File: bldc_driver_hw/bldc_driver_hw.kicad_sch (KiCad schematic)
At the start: 4 parts, among them J1 USB_C_Receptacle_USB2.0_16P, J2 Conn_01x03_Pin

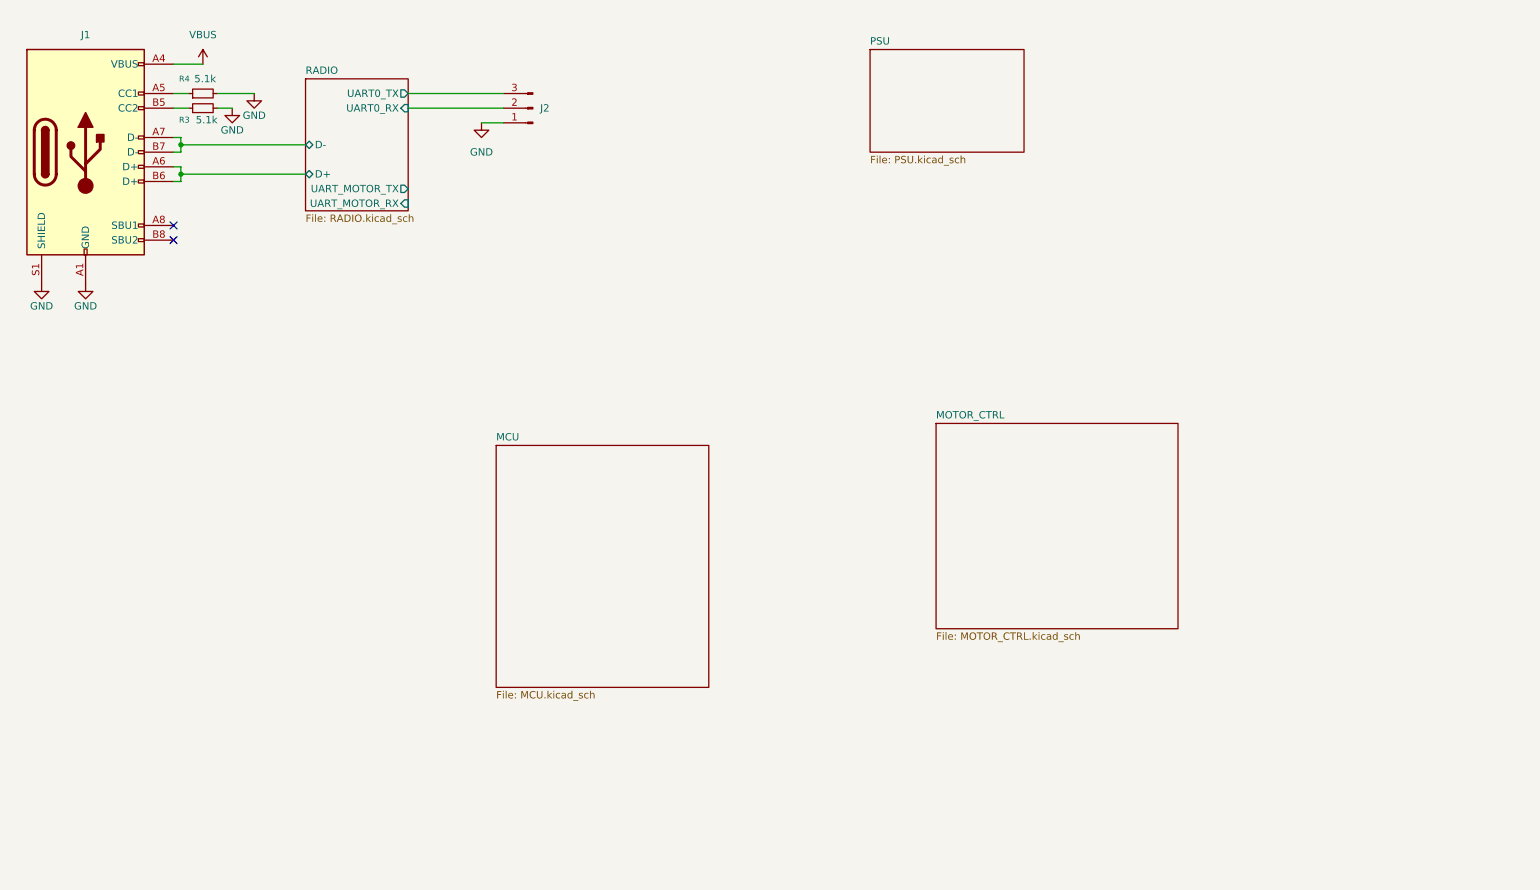
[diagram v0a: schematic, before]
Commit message: wip
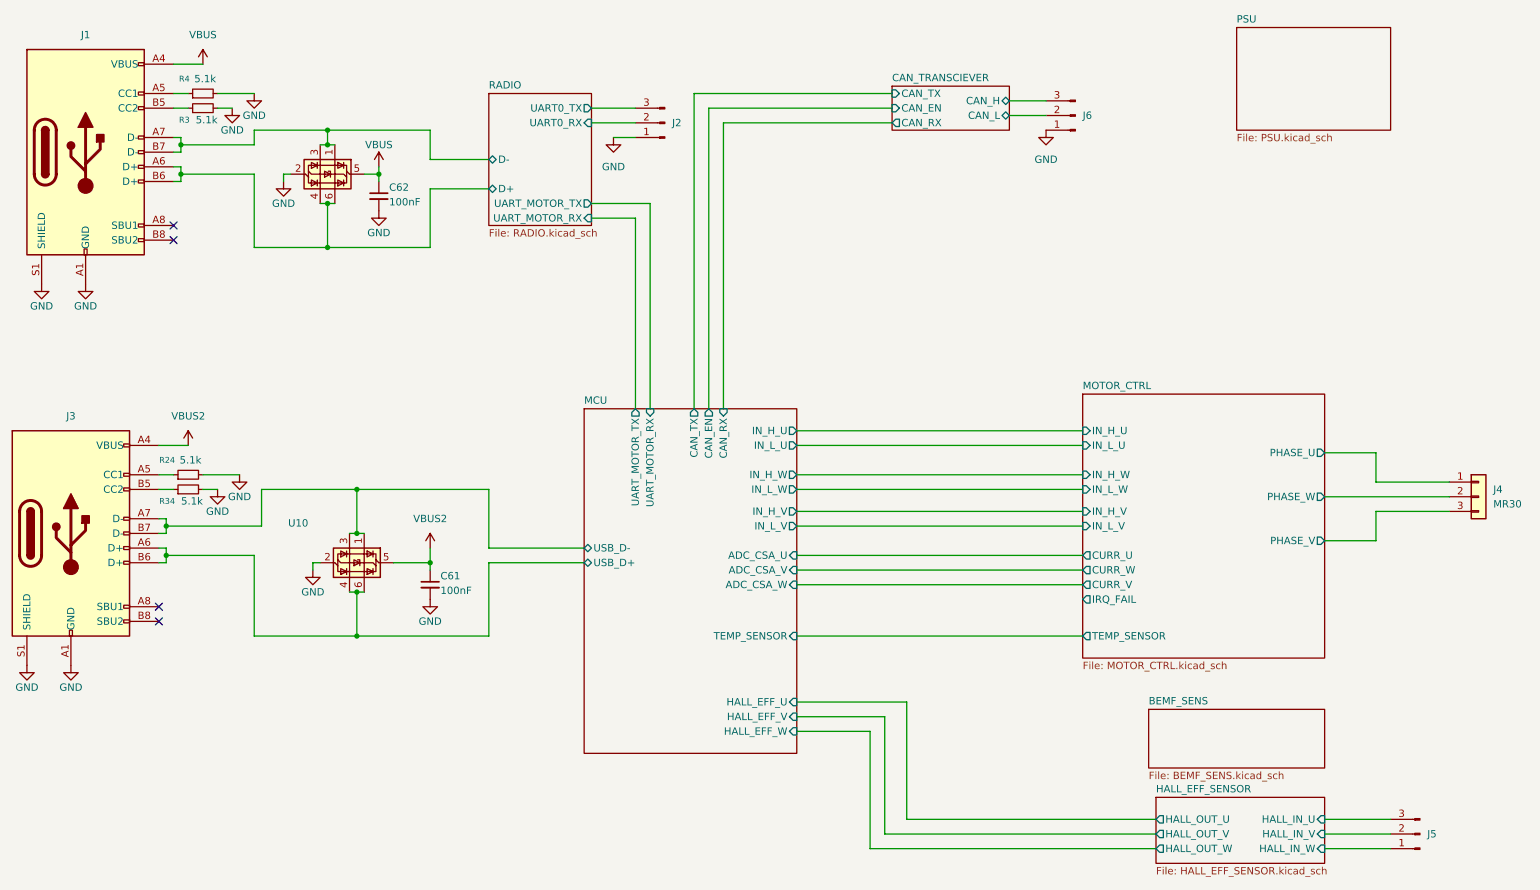
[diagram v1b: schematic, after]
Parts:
- added C61, C62: 100nF, Capacitor_SMD:C_0603_1608Metric, symbol Device:C_Small
- added J3: USB_C_Receptacle_USB2.0_16P, Connector_USB:USB_C_Receptacle_GCT_USB4105-xx-A_16P_TopMnt_Horizontal, symbol Connector:USB_C_Receptacle_USB2.0_16P
- added J4: MR30, Connector_AMASS:AMASS_MR30PW-FB_1x03_P3.50mm_Horizontal, symbol Connector_Generic:Conn_01x03
- added J5, J6: Conn_01x03_Pin, Connector_PinHeader_2.54mm:PinHeader_1x03_P2.54mm_Vertical, symbol Connector:Conn_01x03_Pin
- added R24, R34: 5.1k, Capacitor_SMD:C_0603_1608Metric, symbol Device:R_Small
- added U10, U11: USBLC6-2SC6, Package_TO_SOT_SMD:SOT-23-6, symbol Power_Protection:USBLC6-2SC6
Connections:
- net GND: now also C61.2, C62.2, J3.A1 (GND), J3.A12 (GND), J3.B1 (GND), J3.B12 (GND), J3.S1 (SHIELD), J6.1 (Pin_1), R24.2, R34.2, U10.2 (GND), U11.2 (GND)
- net RADIO/D+: now also U11.4 (I/O2), U11.6 (I/O1)
- net RADIO/D-: now also U11.1 (I/O1), U11.3 (I/O2)
- net VBUS: now also C62.1, U11.5 (VBUS)
- new net: J3.A5 (CC1), R24.1
- new net: J3.B5 (CC2), R34.1
- new net CAN_TRANSCIEVER/CAN_H: J6.3 (Pin_3)
- new net CAN_TRANSCIEVER/CAN_L: J6.2 (Pin_2)
- new net HALL_EFF_SENSOR/HALL_IN_U: J5.3 (Pin_3)
- new net HALL_EFF_SENSOR/HALL_IN_V: J5.2 (Pin_2)
- new net HALL_EFF_SENSOR/HALL_IN_W: J5.1 (Pin_1)
- new net MCU/USB_D+: J3.A6 (D+), J3.B6 (D+), U10.4 (I/O2), U10.6 (I/O1)
- new net MCU/USB_D-: J3.A7 (D-), J3.B7 (D-), U10.1 (I/O1), U10.3 (I/O2)
- new net MOTOR_CTRL/PHASE_U: J4.1 (Pin_1)
- new net MOTOR_CTRL/PHASE_V: J4.3 (Pin_3)
- new net MOTOR_CTRL/PHASE_W: J4.2 (Pin_2)
- new net VBUS2: C61.1, J3.A4 (VBUS), J3.A9 (VBUS), J3.B4 (VBUS), J3.B9 (VBUS), U10.5 (VBUS)
- no-connect marks 2 -> 4
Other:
- added sheet BEMF_SENS (BEMF_SENS.kicad_sch)
- added sheet CAN_TRANSCIEVER (CAN_TRANSCIEVER.kicad_sch)
- added sheet HALL_EFF_SENSOR (HALL_EFF_SENSOR.kicad_sch)
- sheet MCU ports: added ADC_CSA_U, ADC_CSA_V, ADC_CSA_W, CAN_EN, CAN_RX, CAN_TX, HALL_EFF_U, HALL_EFF_V, HALL_EFF_W, IN_H_U, IN_H_V, IN_H_W, IN_L_U, IN_L_V, IN_L_W, TEMP_SENSOR, UART_MOTOR_RX, UART_MOTOR_TX, USB_D+, USB_D-; removed none
- sheet MOTOR_CTRL ports: added CURR_U, CURR_V, CURR_W, IN_H_U, IN_H_V, IN_H_W, IN_L_U, IN_L_V, IN_L_W, IRQ_FAIL, PHASE_U, PHASE_V, PHASE_W, TEMP_SENSOR; removed none
- moved on the sheet: J2
